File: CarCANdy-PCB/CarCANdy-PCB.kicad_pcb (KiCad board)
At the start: 2 copper layers, 101.8 x 68.5 mm, 78 parts, among them J1 8P8C_Shielded, J2 Power, J3 TB004-508-03BE, J4 AUART1, J5 TB004-508-03BE, J6 TB004-508-03BE, J7 TB004-508-03BE, J8 AUART1, J9 TB004-508-03BE, K3 IM02, K4 IM02, K5 IM02, Q1 AO3400A, Q2 AO3400A, Q3 AO3400A, SW2 JS202011CQN, SW3 JS202011CQN, SW4 JS202011CQN, U1 LTV-357T, U2 ESP32-C3_SUPERMINI_TH, U3 SN65HVD233DR, U4 SN65HVD233DR, U5 SN65HVD233DR, U6 Teensy4.1, U7 LTV-357T, U8 LTV-357T

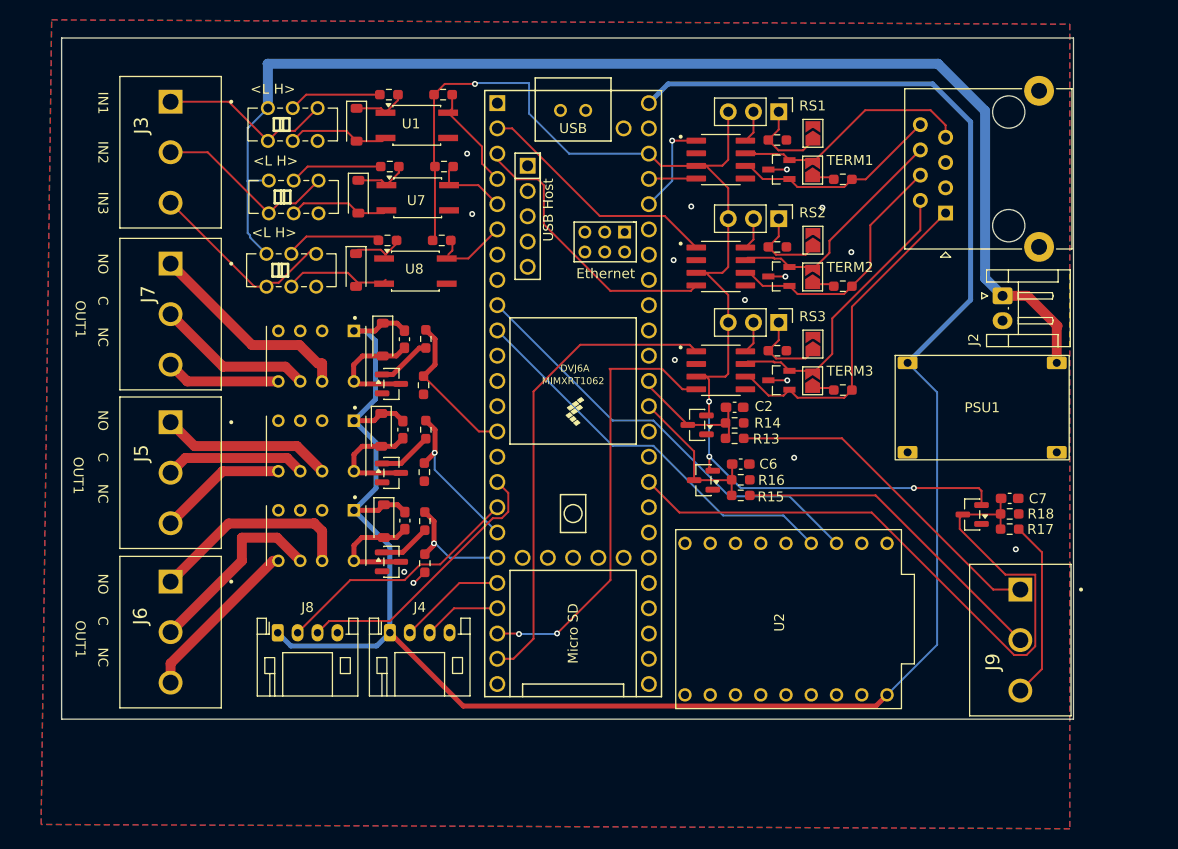
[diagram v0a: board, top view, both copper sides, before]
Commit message: added to PCB
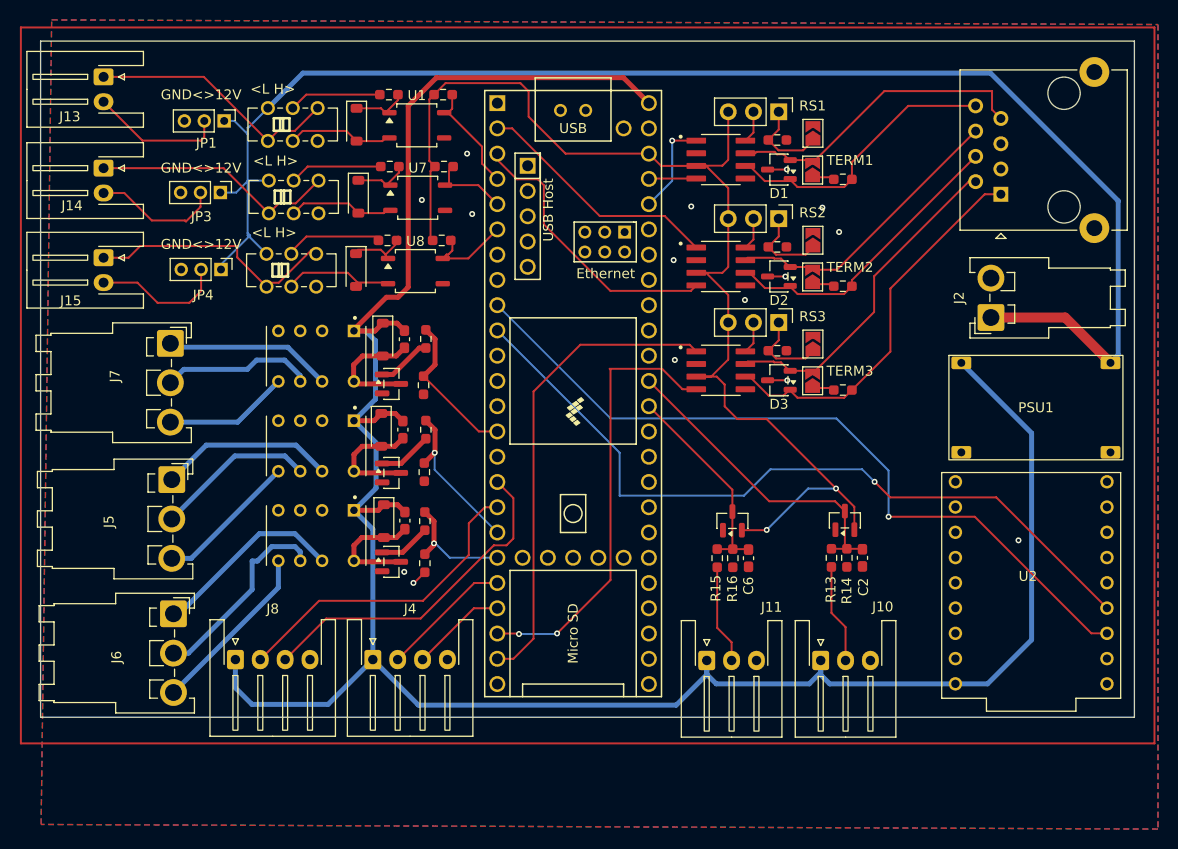
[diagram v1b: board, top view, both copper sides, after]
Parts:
- removed C7: 100nF, Capacitor_SMD:C_0603_1608Metric_Pad1.08x0.95mm_HandSolder
- removed D14: BAT54S, Package_TO_SOT_SMD:SOT-23
- removed J3, J9: TB004-508-03BE, TB004-508-03BE:CUI_TB004-508-03BE
- removed R17: 22K, Resistor_SMD:R_0603_1608Metric_Pad0.98x0.95mm_HandSolder
- removed R18: 33K, Resistor_SMD:R_0603_1608Metric_Pad0.98x0.95mm_HandSolder
- added J10: ADC1, Connector_JST:JST_XH_S3B-XH-A-1_1x03_P2.50mm_Horizontal, F.Cu at (131.0, 111.9)
- added J11: ADC1, Connector_JST:JST_XH_S3B-XH-A-1_1x03_P2.50mm_Horizontal, F.Cu at (119.6, 111.9)
- added J13: Conn_01x02_Pin, Connector_JST:JST_XH_S2B-XH-A-1_1x02_P2.50mm_Horizontal, F.Cu at (58.9, 53.2)
- added J14: Conn_01x02_Pin, Connector_JST:JST_XH_S2B-XH-A-1_1x02_P2.50mm_Horizontal, F.Cu at (58.9, 62.4)
- added J15: Conn_01x02_Pin, Connector_JST:JST_XH_S2B-XH-A-1_1x02_P2.50mm_Horizontal, F.Cu at (58.9, 71.4)
- added JP1: VSEL, Connector_PinHeader_2.00mm:PinHeader_1x03_P2.00mm_Vertical, F.Cu at (71.0, 57.6)
- added JP3: VSEL, Connector_PinHeader_2.00mm:PinHeader_1x03_P2.00mm_Vertical, F.Cu at (70.7, 64.8)
- added JP4: VSEL, Connector_PinHeader_2.00mm:PinHeader_1x03_P2.00mm_Vertical, F.Cu at (70.7, 72.5)
- D1, D2, D3: footprint nup2105lt1g:SOT95P237X111-3N -> Package_TO_SOT_SMD:SOT-23-3
- J2: footprint Connector_JST:JST_EH_S2B-EH_1x02_P2.50mm_Horizontal -> Connector_JST:JST_VH_S2P-VH_1x02_P3.96mm_Horizontal
- J4, J8: footprint Connector_JST:JST_PH_S4B-PH-K_1x04_P2.00mm_Horizontal -> Connector_JST:JST_XH_S4B-XH-A-1_1x04_P2.50mm_Horizontal
- J5, J6, J7: value TB004-508-03BE -> JSTVH3; footprint TB004-508-03BE:CUI_TB004-508-03BE -> Connector_JST:JST_VH_S3P-VH_1x03_P3.96mm_Horizontal
- U1, U7, U8: footprint Package_SO:SO-4_4.4x3.6mm_P2.54mm -> Package_SO:SOP-4_3.8x4.1mm_P2.54mm
- moved U2 24.6 mm to (152.2, 104.3), turned to 180 degrees
- moved C2 19.9 mm to (135.2, 101.5), turned to -90 degrees
- moved D7 17.7 mm to (133.5, 97.8), turned to 90 degrees
- moved R14 17.7 mm to (133.7, 101.5), turned to -90 degrees
- moved R13 15.5 mm to (132.1, 101.5), turned to 90 degrees
- moved C6 9.49 mm to (123.8, 101.6), turned to -90 degrees
- moved J7 8.02 mm to (65.6, 80.0)
- moved R16 7.92 mm to (122.2, 101.6), turned to -90 degrees
- moved R15 6.74 mm to (120.6, 101.6), turned to 90 degrees
- moved J1 5.87 mm to (149.2, 65.0)
- moved J5 5.77 mm to (65.8, 93.7)
- moved PSU1 5.40 mm to (152.7, 86.4)
- moved J8 5.04 mm to (72.2, 111.8)
- moved D13 5.02 mm to (122.2, 97.8), turned to 90 degrees
- moved J6 3.24 mm to (65.9, 107.2)
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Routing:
- net ADC3: track 71.6 -> 0.00 mm
- net T_TX->E_RX: track 40.4 -> 77.6 mm, vias 0 -> 1
- net T_RX->E_TX: track 44.0 -> 77.7 mm, vias 0 -> 1
- net +12V: track 126.9 -> 152.3 mm
- net 5V_SIG1: track 34.1 -> 10.00 mm
- net 5V_SIG2: track 33.2 -> 9.98 mm
- net ADC1: track 13.8 -> 32.1 mm
- net 5V_SIG3: track 18.1 -> 0.00 mm
- net +5V: track 217.3 -> 235.1 mm
- net Net-(J13-Pin_2): track 0.00 -> 13.5 mm
- net Net-(J15-Pin_2): track 0.00 -> 13.3 mm
- net Net-(J14-Pin_2): track 0.00 -> 13.0 mm
- net 12V_SELECT_INPUT1: track 17.8 -> 25.6 mm
- net CAN1_L: track 21.1 -> 28.4 mm
- net CAN1_H: track 24.6 -> 31.4 mm
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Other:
- board size 101.8 x 68.5 mm -> 110 x 68 mm
- board text added: "GND<>12V"
- board text removed: "IN1"
- board text removed: "IN2"
- board text removed: "IN3"
- board text removed: "NO C NC"
- board text removed: "OUT1"
